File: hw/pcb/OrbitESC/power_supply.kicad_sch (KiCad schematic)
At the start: 30 parts, among them J11 VDC, J12 GND, Q7 2N7002, U7 AP62200Z6-7, U8 AP2171W, U9 AP2120

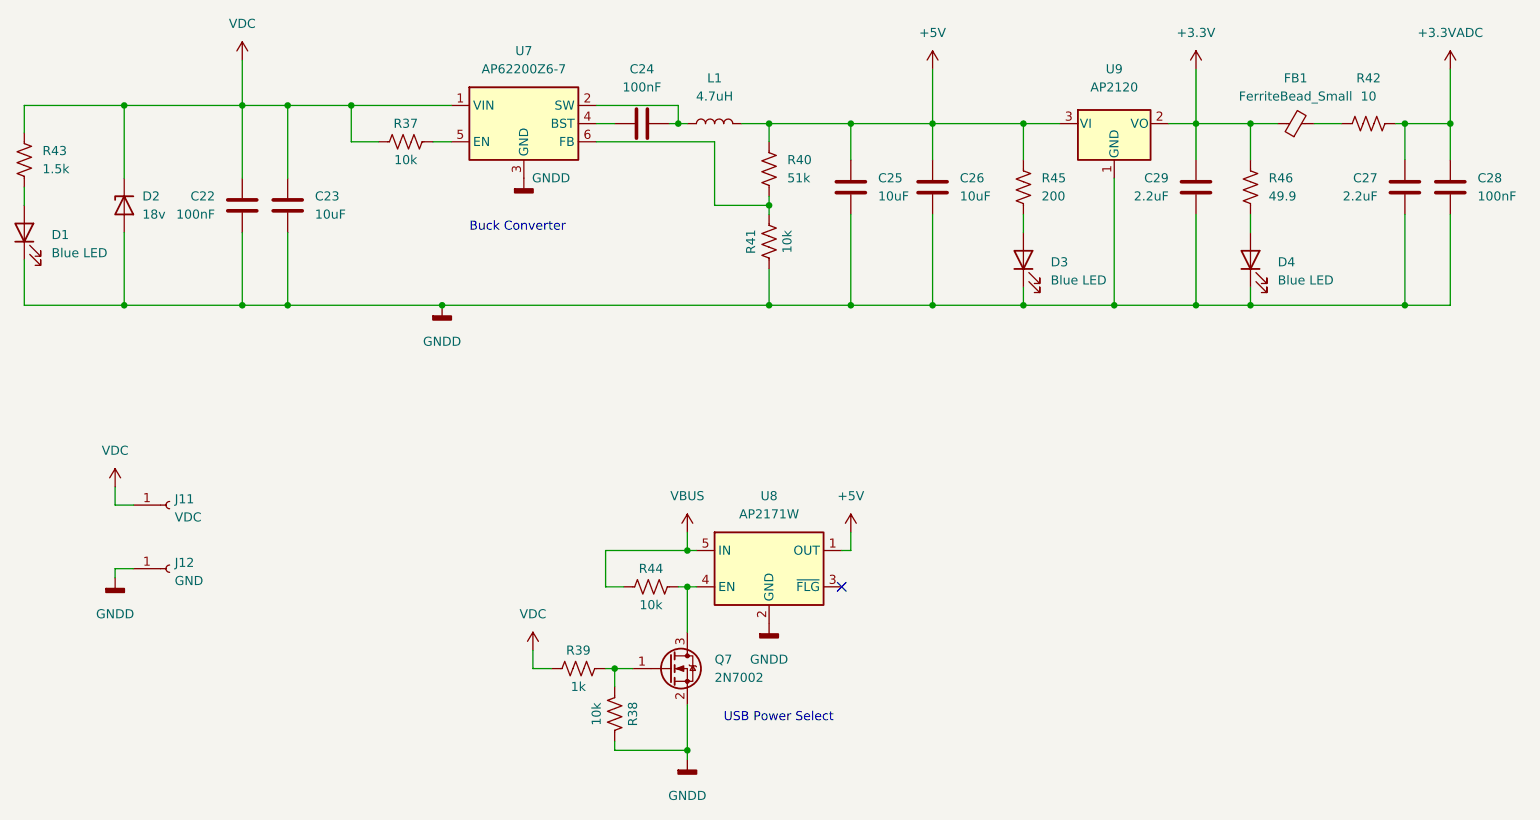
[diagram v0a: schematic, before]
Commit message: Squash feature/sync_current_ctrl/r0
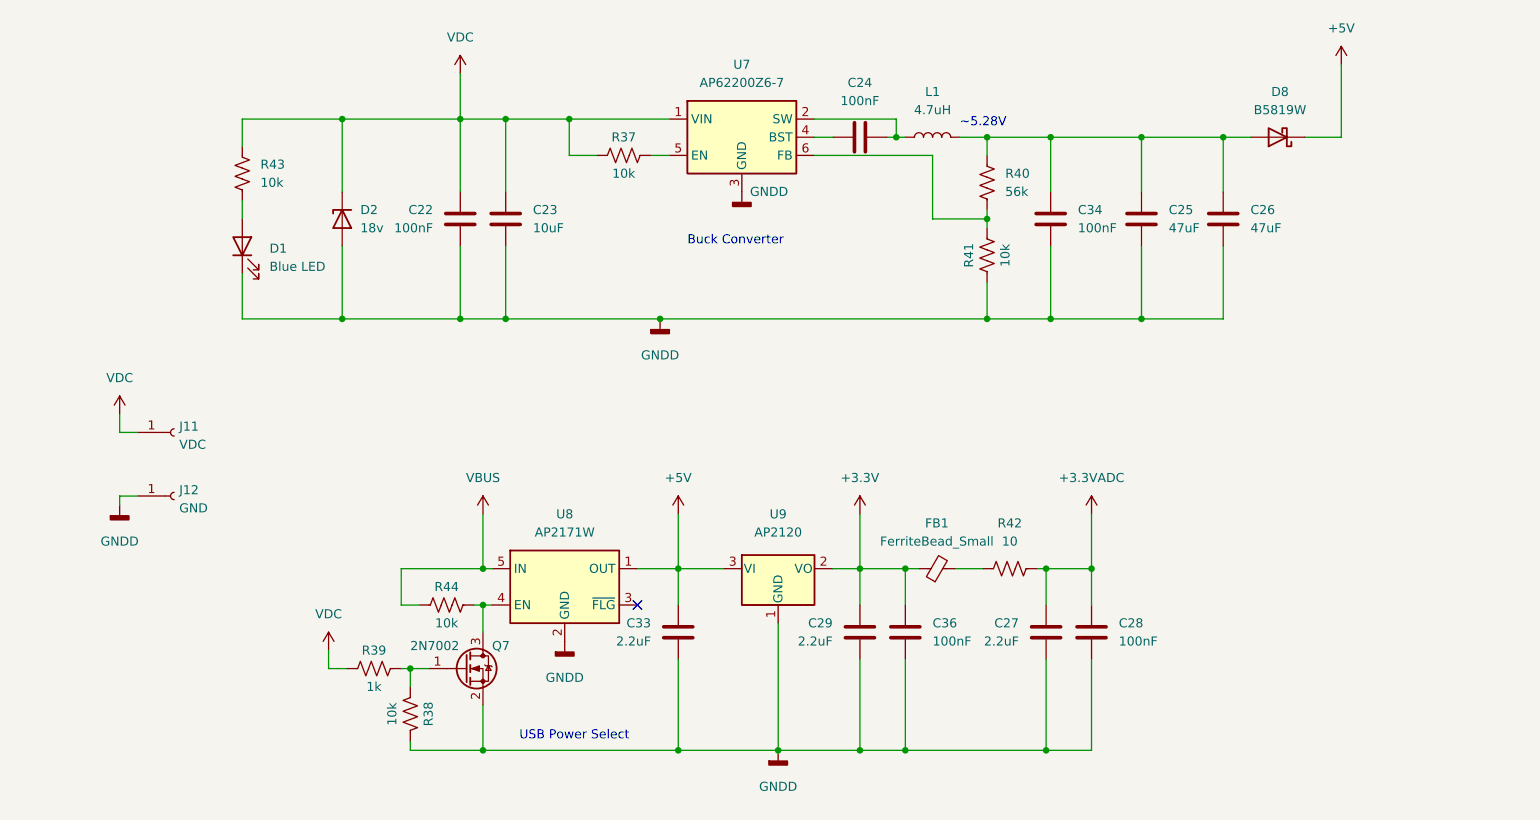
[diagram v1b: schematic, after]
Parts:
- removed D3, D4: Blue LED, Diode_SMD:D_0603_1608Metric, symbol Device:LED
- removed R45: 200, Resistor_SMD:R_0402_1005Metric, symbol Device:R_US
- removed R46: 49.9, Resistor_SMD:R_0402_1005Metric, symbol Device:R_US
- added C33: 2.2uF, Capacitor_SMD:C_0805_2012Metric, symbol Device:C
- added C34, C36: 100nF, Capacitor_SMD:C_0402_1005Metric, symbol Device:C
- added D8: B5819W, Diode_SMD:D_SOD-123, symbol Device:D_Schottky
- C22, C24, C28: JLCPCB C307331 -> (none); LCSC (none) -> C307331
- C23: JLCPCB C440198 -> (none); LCSC (none) -> C440198
- C25, C26: value 10uF -> 47uF; JLCPCB C440198 -> (none); LCSC (none) -> C16780
- C27, C29: JLCPCB C49217 -> (none); LCSC (none) -> C49217
- D1: JLCPCB C72041 -> (none); LCSC (none) -> C72041
- FB1: JLCPCB C1002 -> (none); LCSC (none) -> C1002
- Q7: JLCPCB C8545 -> (none); LCSC (none) -> C8545
- R37, R38, R41, R44: JLCPCB C25744 -> (none); LCSC (none) -> C25744
- R39: JLCPCB C11702 -> (none); LCSC (none) -> C11702
- R40: value 51k -> 56k; DigiKey (none) -> RMCF0402FT57K6CT-ND; JLCPCB C25794 -> (none); LCSC (none) -> C25796
- R42: JLCPCB C25077 -> (none); LCSC (none) -> C25077
- R43: value 1.5k -> 10k; JLCPCB C25867 -> (none); LCSC (none) -> C25744
- U7: LCSC (none) -> C2158024
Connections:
- net +3.3V: now also C36.1
- net +5V: now also C33.2, D8.1 (K); no longer C25.1, C26.1, L1.2, R40.1
- net GNDD: now also C33.1, C34.2, C36.2
- new net: C25.1, C26.1, C34.1, D8.2 (A), L1.2, R40.1
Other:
- note added: "~5.28V"
- moved on the sheet: C22, C23, C24, C25, C26, C27, C28, C29, D1, D2, FB1, J11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
